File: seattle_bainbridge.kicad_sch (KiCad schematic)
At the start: 12 parts

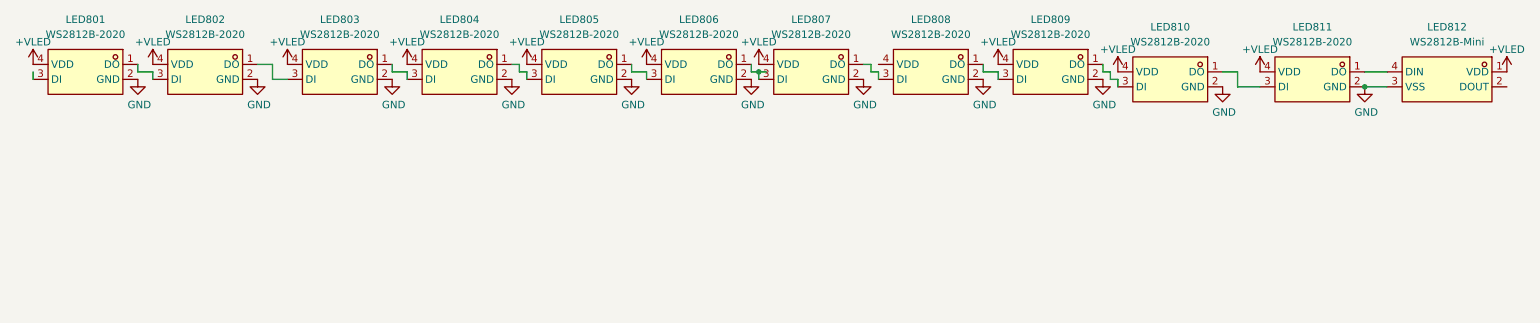
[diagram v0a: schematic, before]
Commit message: junction checkpoint
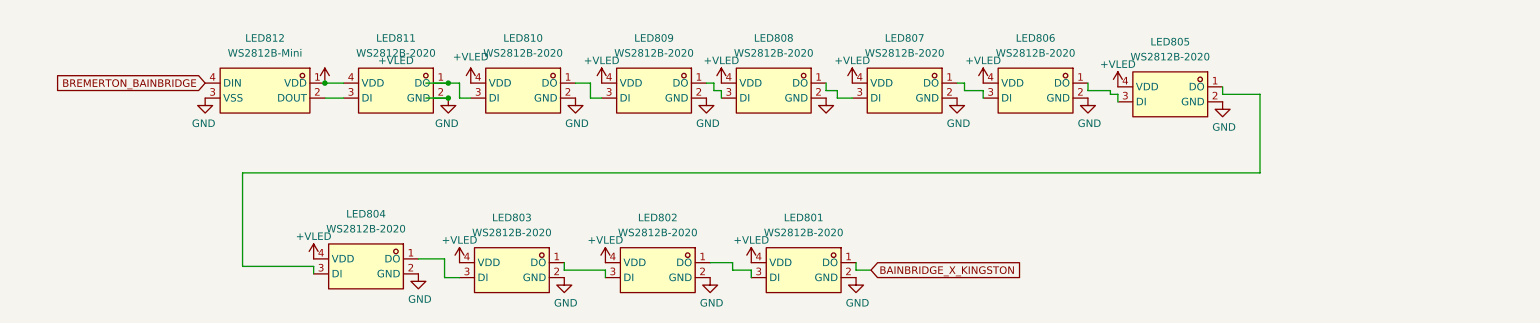
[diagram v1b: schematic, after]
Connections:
- net +VLED: now also LED808.4 (VDD)
- net at LED802.3 (DI): now also LED803.1 (DO); no longer LED801.1 (DO)
- net at LED801.3 (DI): now also LED802.1 (DO)
- net at LED811.1 (DO): now also LED810.3 (DI); no longer LED812.4 (DIN)
- net at LED810.1 (DO): now also LED809.3 (DI); no longer LED811.3 (DI)
- net at LED804.1 (DO): now also LED803.3 (DI); no longer LED805.3 (DI)
- net at LED804.3 (DI): now also LED805.1 (DO); no longer LED803.1 (DO)
- net at LED809.1 (DO): now also LED808.3 (DI); no longer LED810.3 (DI)
- net at LED812.2 (DOUT): now also LED811.3 (DI)
- net at LED808.1 (DO): now also LED807.3 (DI); no longer LED809.3 (DI)
- net at LED807.1 (DO): now also LED806.3 (DI); no longer LED808.3 (DI)
- net at LED806.1 (DO): now also LED805.3 (DI); no longer LED807.3 (DI)
- new net BAINBRIDGE_X_KINGSTON: LED801.1 (DO)
- new net BREMERTON_BAINBRIDGE: LED812.4 (DIN)
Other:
- moved on the sheet: LED801, LED810, LED811, LED812
